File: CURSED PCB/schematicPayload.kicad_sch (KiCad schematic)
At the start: 25 parts, among them J1 Conn_01x02, J2 SD_Card_Device, J3 Conn_PIC_ICSP_ICD, U1 LT1962-3.3, U10 MAX1968xUI, U11 AD9850, U12 LTC6102HVxDD, U13 LTC3886, U14 CY7C65213-28PVXI, U15 ESD224DQA, U2 STM32F401CBUx, U3 OPA847xD, U4 TVS0500DRV, U5 LM4132xMF-1.8, U6 BUF602xD, U7 ADC082S021, U8 LPF-B0R3, U9 iC-HTG

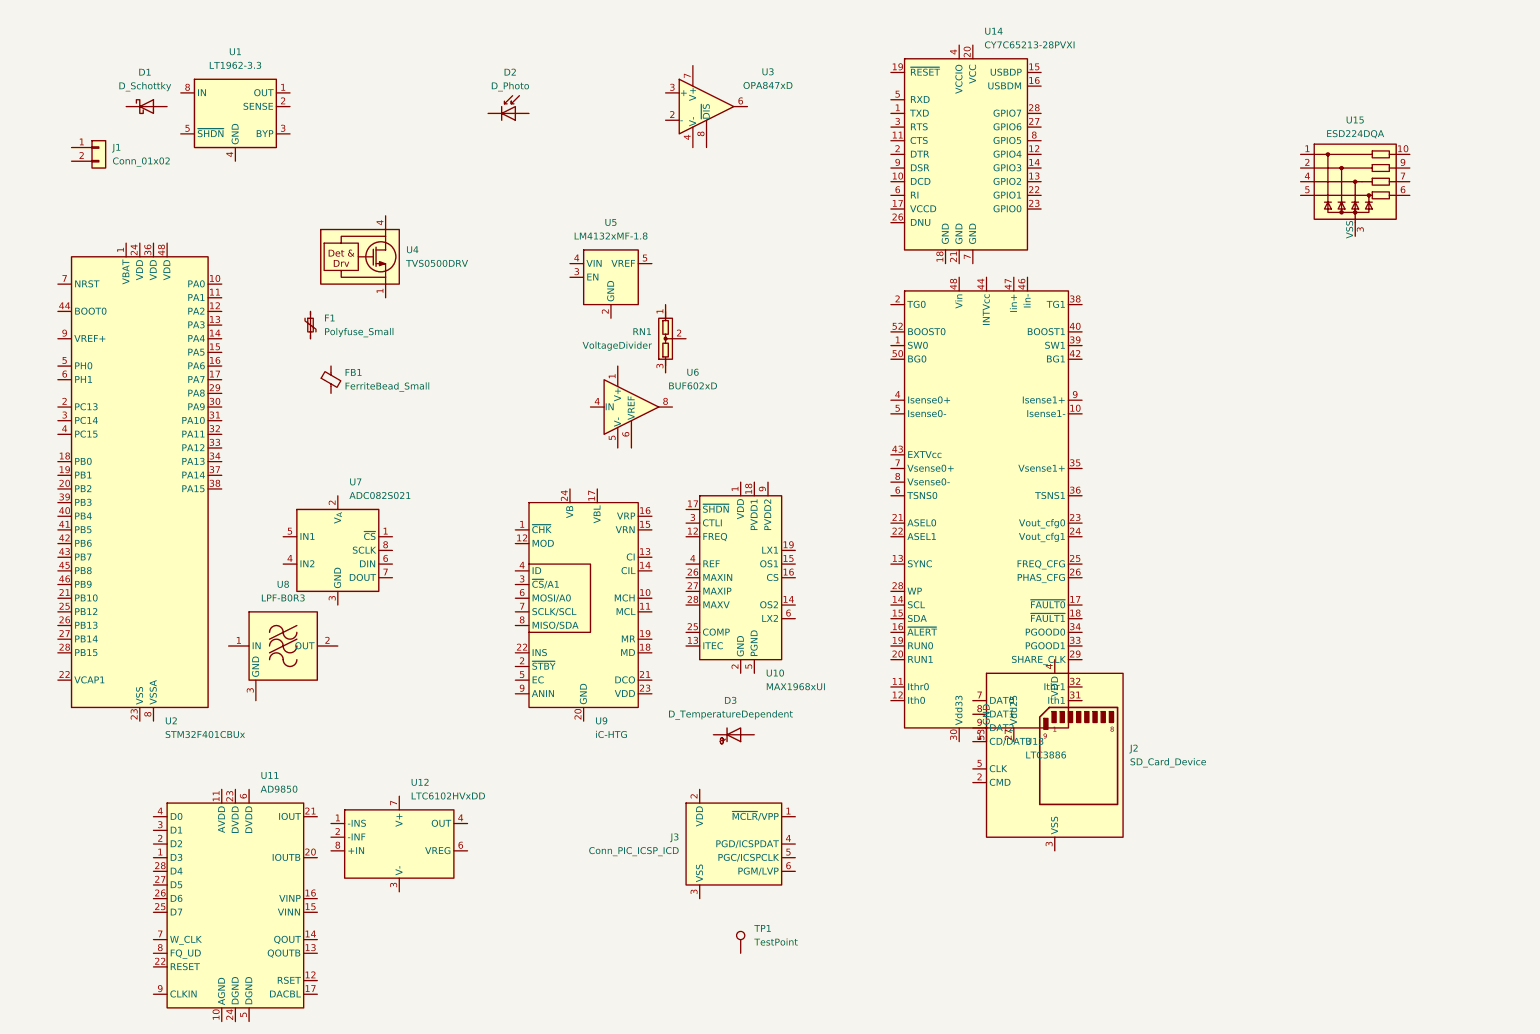
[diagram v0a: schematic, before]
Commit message: added stuff
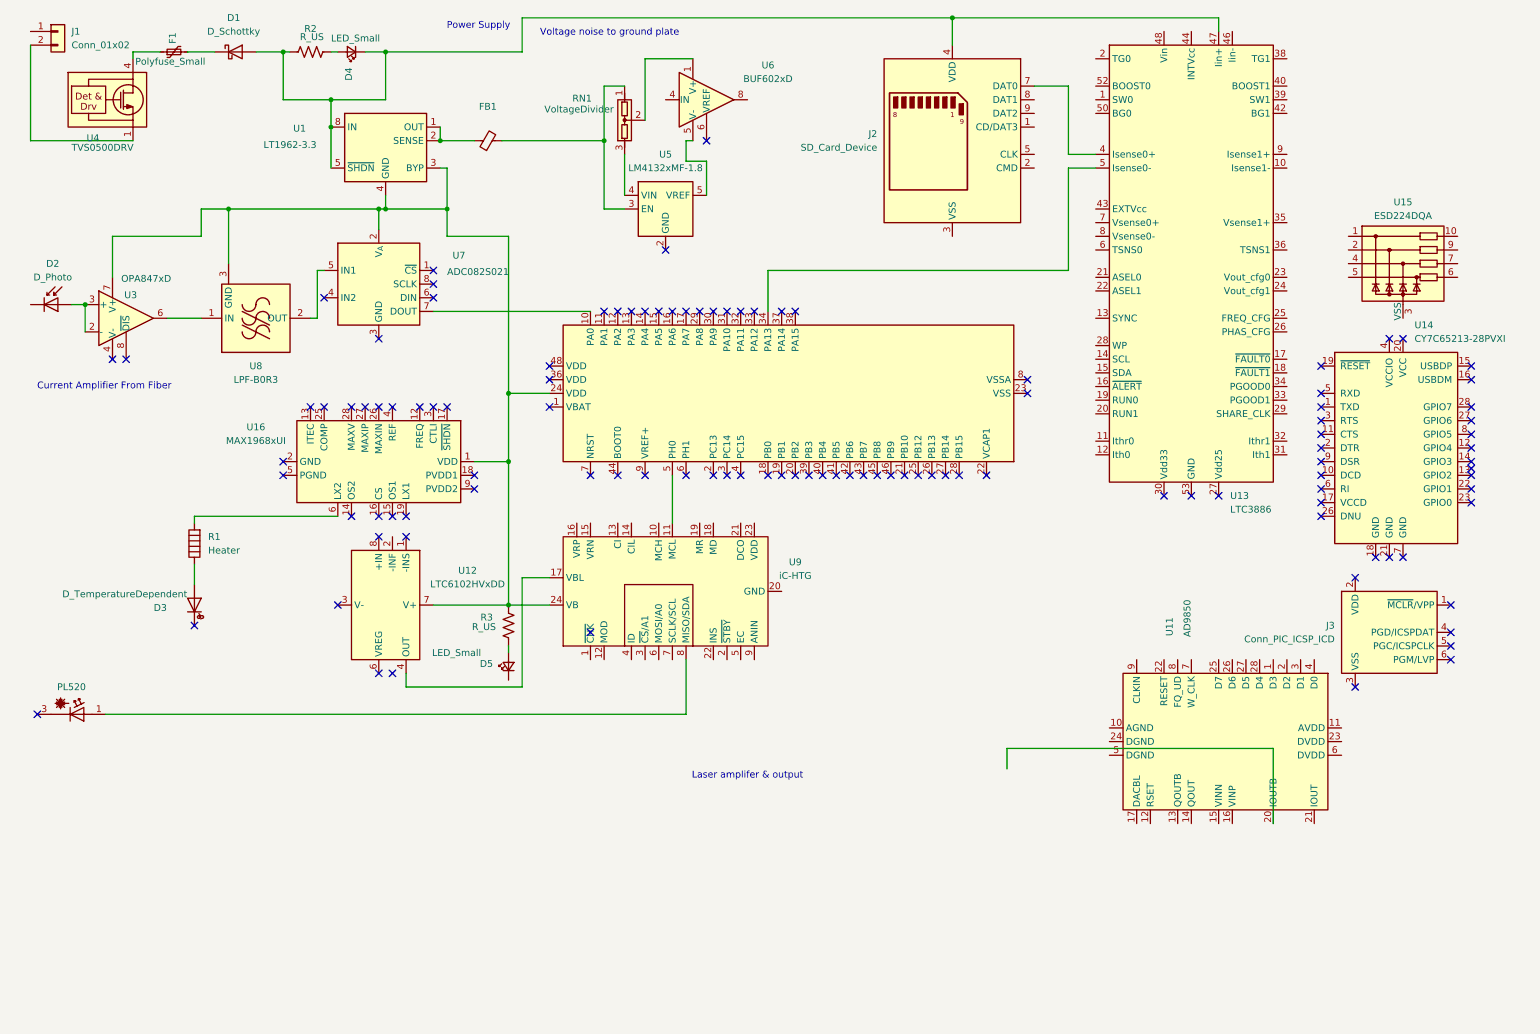
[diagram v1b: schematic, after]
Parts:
- removed TP1: TestPoint, symbol Connector:TestPoint
- removed U10: MAX1968xUI, Package_SO:HTSSOP-28-1EP_4.4x9.7mm_P0.65mm_EP2.85x5.4mm, symbol Driver_TEC:MAX1968xUI
- added D4, D5: LED_Small, symbol Device:LED_Small
- added LD1: PL520, OptoDevice:LaserDiode_TO38ICut-3, symbol Diode_Laser:PL520
- added R1: Heater, symbol Device:Heater
- added R2, R3: R_US, symbol Device:R_US
- added U16: MAX1968xUI, Package_SO:HTSSOP-28-1EP_4.4x9.7mm_P0.65mm_EP2.85x5.4mm, symbol Driver_TEC:MAX1968xUI
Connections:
- net at U8.1 (IN): now also U3.6
- net at U8.2 (OUT): now also U7.5 (IN1)
- net at U8.3 (GND), U8.4 (GND), U8.5 (GND)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: now also U1.3 (BYP), U1.4 (GND), U12.7 (V+), U2.24 (VDD), U3.7 (V+), U7.2 (V_{A}), U9.24 (VB), R3.1, U16.1 (VDD)
- net at RN1.1: now also FB1.2, U5.3 (EN)
- net at RN1.2: now also U6.1 (V+)
- net at RN1.3: now also U5.4 (VIN)
- net at J2.4 (VDD): now also D1.2 (A), U1.5 (~{SHDN}), U1.8 (IN), U13.47 (Iin+), D4.1 (K), R2.1
- net at J2.7 (DAT0): now also U13.4 (Isense0+)
- net at U12.4 (OUT): now also U9.17 (VBL)
- net at D1.1 (K): now also F1.2
- net at U1.1 (OUT): now also FB1.1, U1.2 (SENSE)
- net at U5.5 (VREF): now also U6.5 (V-)
- net at U7.7 (DOUT): now also U2.10 (PA0)
- net at J1.2 (Pin_2): now also U4.1 (GND), U4.2 (GND), U4.3 (GND), U4.7 (GND)
- net at U2.34 (PA13): now also U13.5 (Isense0-)
- net at U2.5 (PH0): now also U9.11 (MCL)
- net at D2.2 (A): now also U3.2 (-), U3.3 (+)
- net at D3.2 (A): now also R1.1
- net at F1.1: now also U4.4 (IN), U4.5 (IN), U4.6 (IN)
- net at U9.8 (MISO/SDA): now also LD1.1 (A)
- new net: D4.2 (A), R2.2
- new net: D5.2 (A), R3.2
- new net: R1.2, U16.10 (LX2), U16.6 (LX2), U16.8 (LX2)
- new net: U16.11 (PVDD2), U16.9 (PVDD2)
- new net: U16.18 (PVDD1), U16.20 (PVDD1)
- new net: U16.19 (LX1), U16.21 (LX1), U16.23 (LX1)
- new net: U16.2 (GND), U16.29 (GND)
- new net: U16.22 (PGND), U16.24 (PGND), U16.5 (PGND), U16.7 (PGND)
- no-connect marks 0 -> 112
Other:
- note added: "Current Amplifier From Fiber"
- note added: "Laser amplifer & output"
- note added: "Power Supply"
- note added: "Voltage noise to ground plate"
- moved on the sheet: D1, D2, D3, F1, FB1, J1, J2, J3, RN1, U1, U11, U12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
